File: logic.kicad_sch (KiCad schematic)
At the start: 5 parts, among them IC4 74AHC1G08GW-Q100,1, IC5 74HC14PW-Q100,118

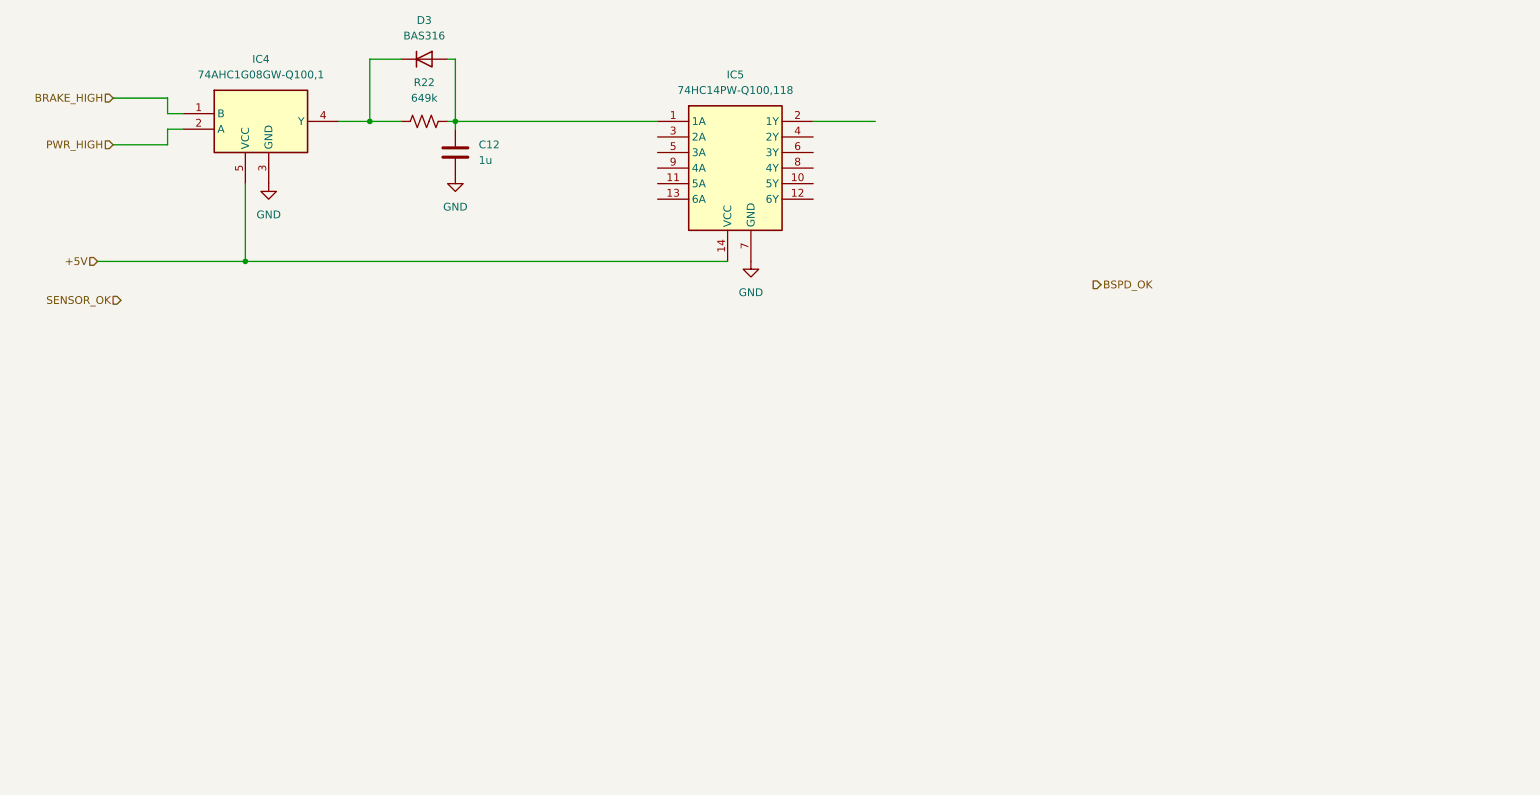
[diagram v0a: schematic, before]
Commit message: Latch and reset started
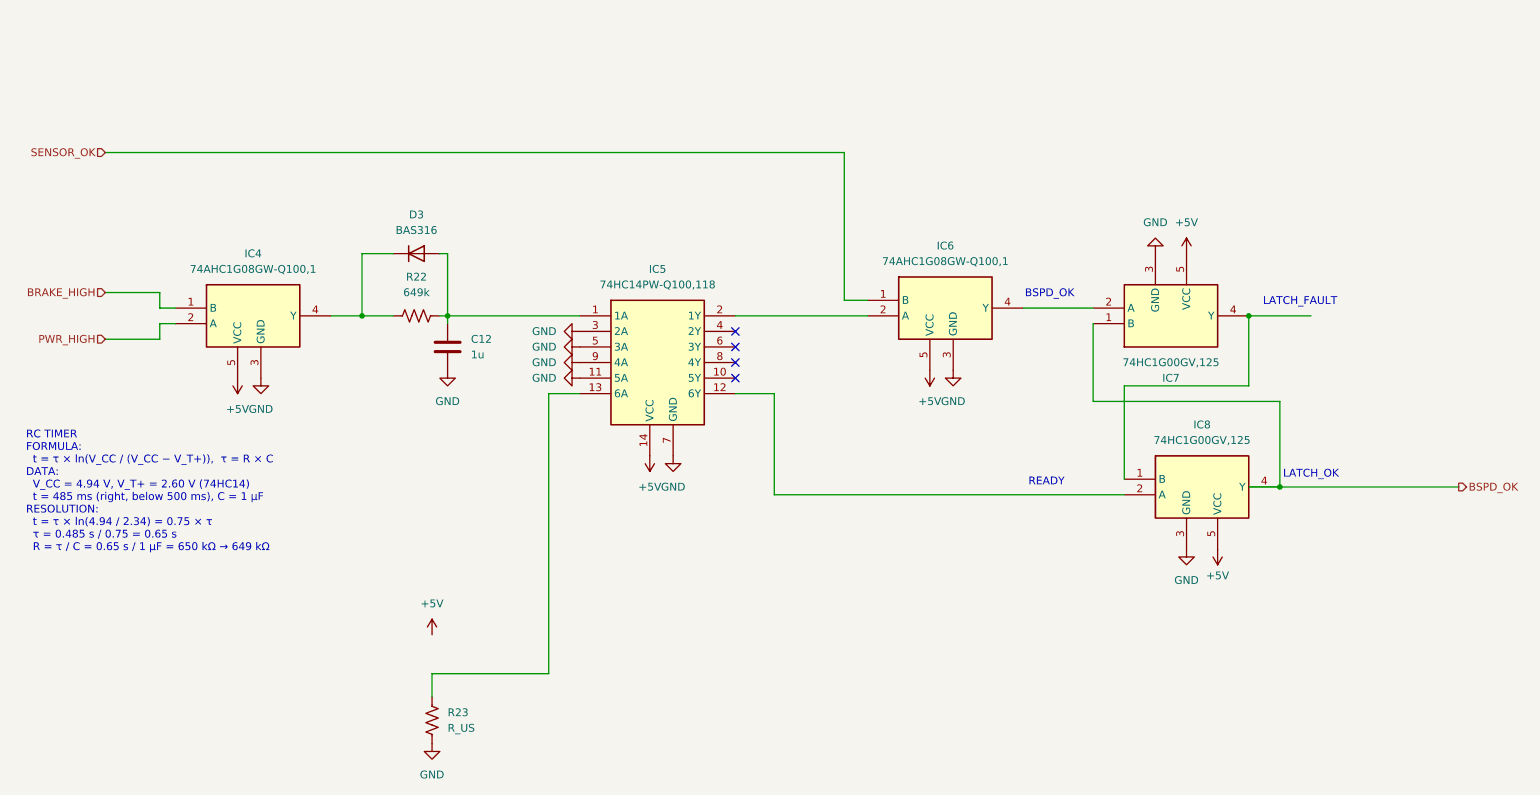
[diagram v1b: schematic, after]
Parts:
- added IC6: 74AHC1G08GW-Q100,1, SOT65P212X110-5N, symbol SamacSys:74AHC1G08GW-Q100,1
- added IC7, IC8: 74HC1G00GV,125, SOT95P275X110-5N, symbol SamacSys:74HC1G00GV,125
- added R23: R_US, Resistor_SMD:R_0603_1608Metric, symbol Device:R_US
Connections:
- net +5V: now also IC6.5 (VCC), IC7.5 (VCC), IC8.5 (VCC)
- net BSPD_OK: now also IC7.1 (B), IC8.4 (Y)
- net GND: now also IC5.11 (5A), IC5.3 (2A), IC5.5 (3A), IC5.9 (4A), IC6.3 (GND), IC7.3 (GND), IC8.3 (GND), R23.2
- net SENSOR_OK: now also IC6.1 (B)
- net at IC5.12 (6Y): now also IC8.2 (A)
- net at IC5.13 (6A): now also R23.1
- net at IC5.2 (1Y): now also IC6.2 (A)
- new net: IC7.4 (Y), IC8.1 (B)
- new net: IC6.4 (Y), IC7.2 (A)
- no-connect marks 0 -> 4
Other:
- note added: "BSPD_OK"
- note added: "LATCH_FAULT"
- note added: "LATCH_OK"
- note added: "RC TIMER FORMULA: t = τ × ln(V_CC / (V_CC − V_T+)), τ = R × C DATA: V_CC = 4.94 V, V_T+ = 2.60 V (74HC14) t = 485 ms (right, below 500 ms), C = 1 µF RESOLUTION: t = τ × ln(4.94 / 2.34) = 0.75 × τ τ = 0.485 s / 0.75 = 0.65 s R = τ / C = 0.65 s / 1 µF = 650 kΩ → 649 kΩ"
- note added: "READY"
- moved on the sheet: C12, D3, IC4, IC5, R22
